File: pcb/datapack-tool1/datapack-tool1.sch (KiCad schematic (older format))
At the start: 24 parts, among them J1 Conn_01x04_Female, J2 Conn_02x08_Odd_Even, J3 Conn_01x03_Female, M1 P-CHANNEL-MOSFET, SW1 sw, SW2 sw, SW3 sw, U1 Pico, U2 74LS245, U3 74LS245

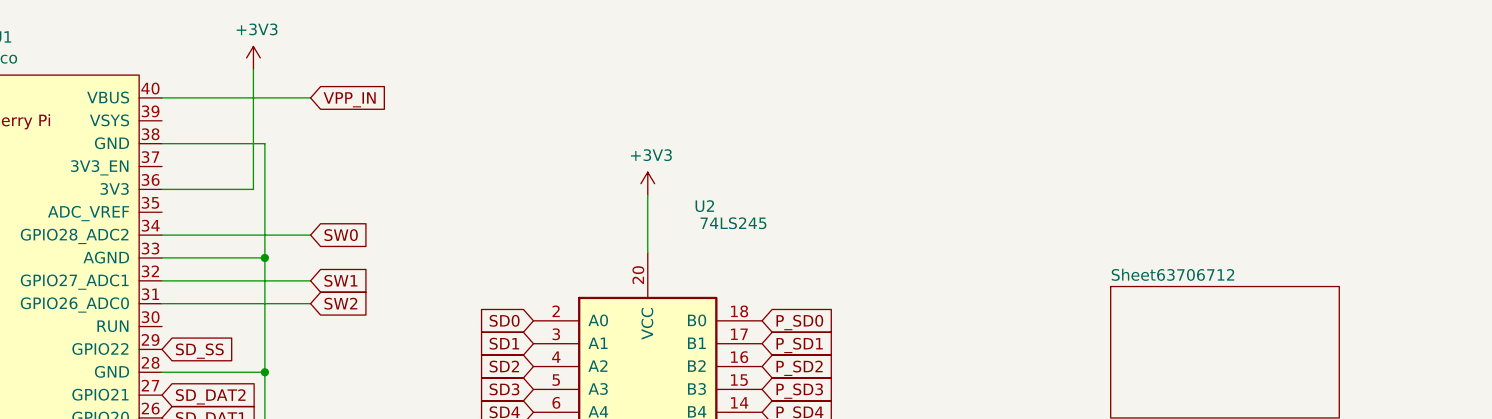
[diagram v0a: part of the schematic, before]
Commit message: Updates
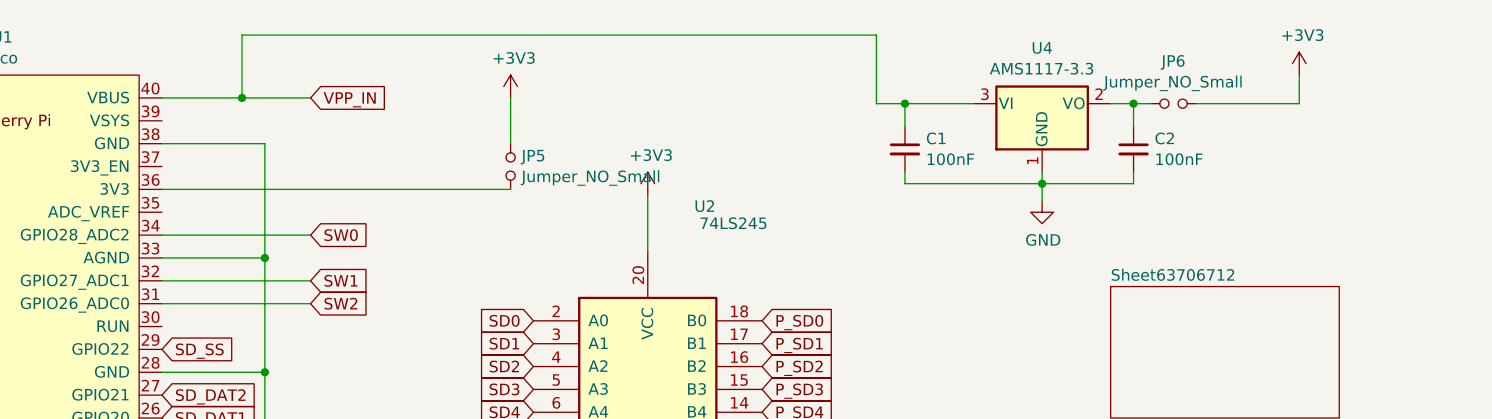
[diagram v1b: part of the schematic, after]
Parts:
- added C1, C2: 100nF, Capacitor_SMD:C_0805_2012Metric, symbol Device:C_Small
- added JP5, JP6: Jumper_NO_Small, Jumper:SolderJumper-2_P1.3mm_Open_TrianglePad1.0x1.5mm, symbol Device:Jumper_NO_Small
- added U4: AMS1117-3.3, Package_TO_SOT_SMD:SOT-223-3_TabPin2, symbol pak_breakout:AMS1117-3.3
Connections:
- net +3V3: now also JP5.1, JP6.2; no longer U1.36 (3V3)
- net GND: now also C1.2, C2.2, U4.1 (GND)
- net VPP_IN: now also C1.1, U4.3 (VI)
- new net: JP5.2, U1.36 (3V3)
- new net: C2.1, JP6.1, U4.2 (VO)
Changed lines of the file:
@@
 L power:GND #PWR0103
 U 1 1 6367C6EB
-P 4850 3250
-F 0 "#PWR0103" H 4850 3000 50  0001 C CNN
-F 1 "GND" H 4855 3077 50  0000 C CNN
-F 2 "" H 4850 3250 50  0001 C CNN
-F 3 "" H 4850 3250 50  0001 C CNN
-	1    4850 3250
+P 6575 1300
+F 0 "#PWR0103" H 6575 1050 50  0001 C CNN
+F 1 "GND" H 6580 1127 50  0000 C CNN
+F 2 "" H 6575 1300 50  0001 C CNN
+F 3 "" H 6575 1300 50  0001 C CNN
+	1    6575 1300
 	1    0    0    -1
 $EndComp
@@
 L power:+3V3 #PWR0105
 U 1 1 6367D4B6
-P 3125 725
-F 0 "#PWR0105" H 3125 575 50  0001 C CNN
-F 1 "+3V3" H 3140 898 50  0000 C CNN
-F 2 "" H 3125 725 50  0001 C CNN
-F 3 "" H 3125 725 50  0001 C CNN
-	1    3125 725
+P 4250 850
+F 0 "#PWR0105" H 4250 700 50  0001 C CNN
+F 1 "+3V3" H 4265 1023 50  0000 C CNN
+F 2 "" H 4250 850 50  0001 C CNN
+F 3 "" H 4250 850 50  0001 C CNN
+	1    4250 850
 	1    0    0    -1
 $EndComp
@@
 	4850 1275 4850 1525
 Wire Wire Line
-	3125 725  3125 1250
-Wire Wire Line
-	3125 1250 2725 1250
+	4250 1250 2725 1250
 Wire Wire Line
 	4850 3125 4850 3250
@@
 VPP_IN
 Wire Wire Line
-	2725 850  3375 850
+	2725 850  3075 850
 Text GLabel 3375 1450 2    50   Input ~ 0
 SW0
@@
 Wire Wire Line
 	975  6975 3000 6975
+$Comp
+L Device:Jumper_NO_Small JP5
+U 1 1 63745F7B
+P 4250 1150
+F 0 "JP5" V 4204 1198 50  0000 L CNN
+F 1 "Jumper_NO_Small" V 4295 1198 50  0000 L CNN
+F 2 "Jumper:SolderJumper-2_P1.3mm_Open_TrianglePad1.0x1.5mm" H 4250 1150 50  0001 C CNN
+F 3 "~" H 4250 1150 50  0001 C CNN
+	1    4250 1150
+	0    1    1    0
+$EndComp
+$Comp
+L Device:Jumper_NO_Small JP6
+U 1 1 63746CAC
+P 7150 875
+F 0 "JP6" H 7150 1060 50  0000 C CNN
+F 1 "Jumper_NO_Small" H 7150 969 50  0000 C CNN
+F 2 "Jumper:SolderJumper-2_P1.3mm_Open_TrianglePad1.0x1.5mm" H 7150 875 50  0001 C CNN
+F 3 "~" H 7150 875 50  0001 C CNN
+	1    7150 875
+	1    0    0    -1
+$EndComp
+Wire Wire Line
+	4250 850  4250 1050
+$Comp
+L pak_breakout:AMS1117-3.3 U4
+U 1 1 6374C131
+P 6575 875
+F 0 "U4" H 6575 1117 50  0000 C CNN
+F 1 "AMS1117-3.3" H 6575 1026 50  0000 C CNN
+F 2 "Package_TO_SOT_SMD:SOT-223-3_TabPin2" H 6575 1075 50  0001 C CNN
+F 3 "" H 6675 625 50  0001 C CNN
+	1    6575 875
+	1    0    0    -1
+$EndComp
+Wire Wire Line
+	6575 1300 6575 1225
+Wire Wire Line
+	6875 875  6975 875
+Wire Wire Line
+	3075 850  3075 575
+Wire Wire Line
+	3075 575  5850 575
+Wire Wire Line
+	5850 575  5850 875
+Wire Wire Line
+	5850 875  5975 875
+Connection ~ 3075 850
+Wire Wire Line
+	3075 850  3375 850
+$Comp
+L power:+3V3 #PWR0123
+U 1 1 6375A2DF
+P 7700 750
+F 0 "#PWR0123" H 7700 600 50  0001 C CNN
+F 1 "+3V3" H 7715 923 50  0000 C CNN
+F 2 "" H 7700 750 50  0001 C CNN
+F 3 "" H 7700 750 50  0001 C CNN
+	1    7700 750
+	1    0    0    -1
+$EndComp
+Wire Wire Line
+	7250 875  7700 875
+Wire Wire Line
+	7700 875  7700 750
+$Comp
+L Device:C_Small C1
+U 1 1 63762D32
+P 5975 1075
+F 0 "C1" H 6067 1121 50  0000 L CNN
+F 1 "100nF" H 6067 1030 50  0000 L CNN
+F 2 "Capacitor_SMD:C_0805_2012Metric" H 5975 1075 50  0001 C CNN
+F 3 "~" H 5975 1075 50  0001 C CNN
+	1    5975 1075
+	1    0    0    -1
+$EndComp
+$Comp
+L Device:C_Small C2
+U 1 1 6376314C
+P 6975 1075
+F 0 "C2" H 7067 1121 50  0000 L CNN
+F 1 "100nF" H 7067 1030 50  0000 L CNN
+F 2 "Capacitor_SMD:C_0805_2012Metric" H 6975 1075 50  0001 C CNN
+F 3 "~" H 6975 1075 50  0001 C CNN
+	1    6975 1075
+	1    0    0    -1
+$EndComp
+Wire Wire Line
+	6975 975  6975 875
+Connection ~ 6975 875
+Wire Wire Line
+	6975 875  7050 875
+Wire Wire Line
+	5975 875  5975 975
+Connection ~ 5975 875
+Wire Wire Line
+	5975 875  6275 875
+Wire Wire Line
+	5975 1175 5975 1225
+Wire Wire Line
+	5975 1225 6575 1225
+Connection ~ 6575 1225
+Wire Wire Line
+	6575 1225 6575 1175
+Wire Wire Line
+	6575 1225 6975 1225
+Wire Wire Line
+	6975 1225 6975 1175
+$Comp
+L power:GND #PWR0124
+U 1 1 637823D8
+P 4850 3250
+F 0 "#PWR0124" H 4850 3000 50  0001 C CNN
+F 1 "GND" H 4855 3077 50  0000 C CNN
+F 2 "" H 4850 3250 50  0001 C CNN
+F 3 "" H 4850 3250 50  0001 C CNN
+	1    4850 3250
+	1    0    0    -1
+$EndComp
 $EndSCHEMATC
